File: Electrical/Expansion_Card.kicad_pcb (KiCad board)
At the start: 2 copper layers, 26 x 30 mm, 50 parts, among them J1 SJ-3501-SMT-TR, J2 SJ-3501-SMT-TR, P1 USB_C_Plug_USB2.0, U2 PCM2906, U3 TPA6132A2RTE, U4 LDLN050PUR, Y1 120-8-36B-CWY-TR

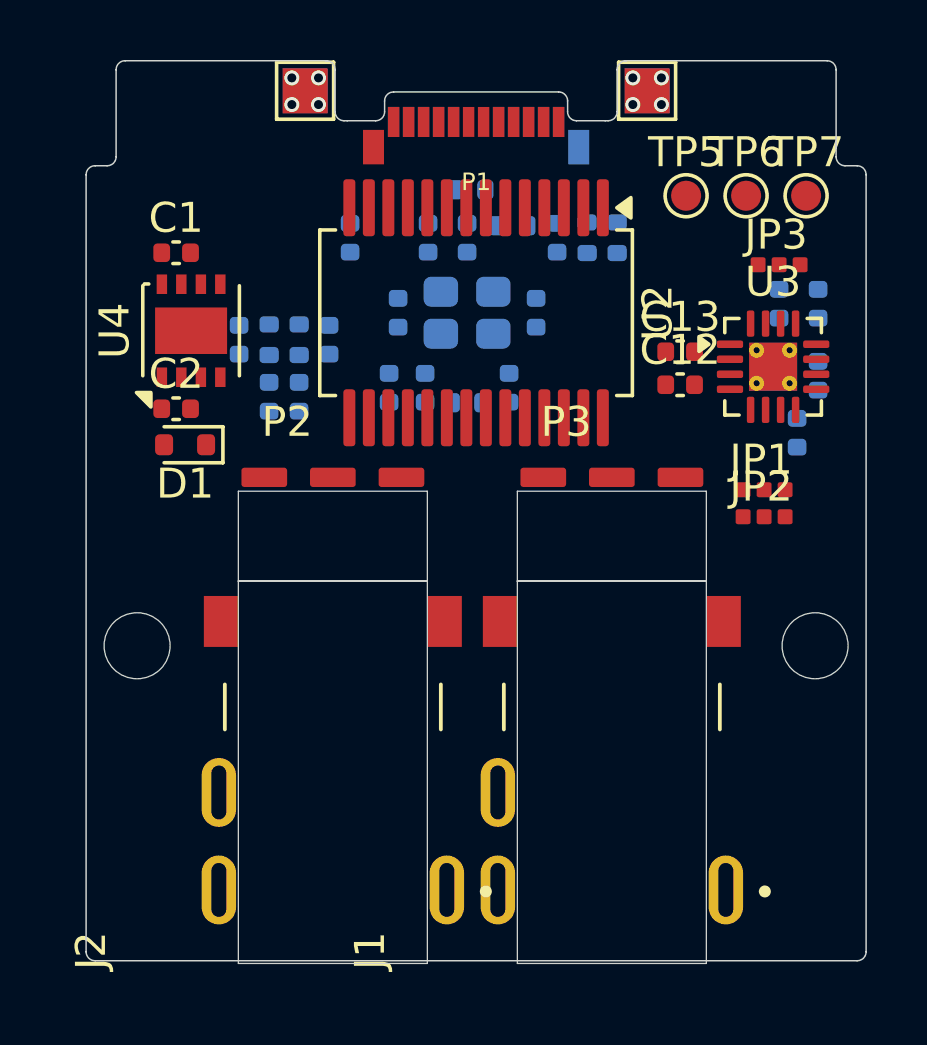
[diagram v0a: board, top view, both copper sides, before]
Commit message: Routing + output
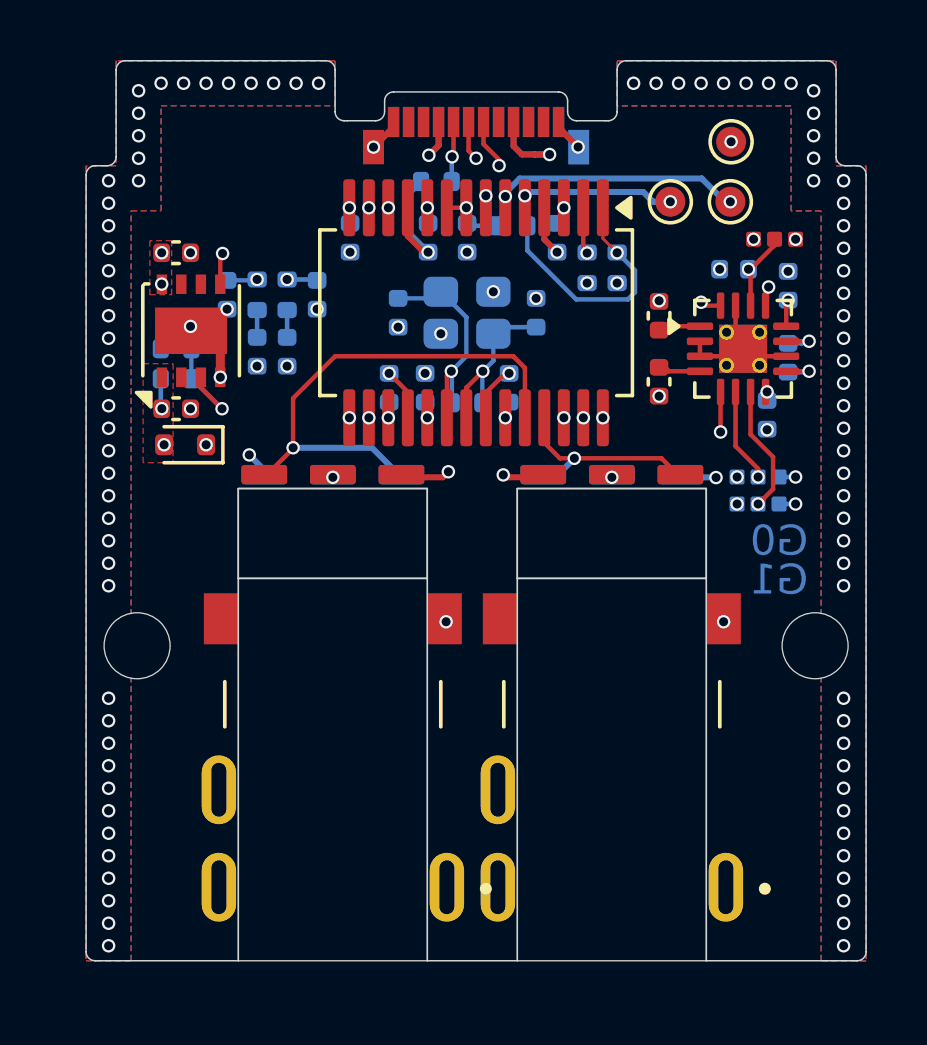
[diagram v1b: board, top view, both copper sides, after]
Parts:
- removed TP1, TP2, TP3, TP4: TestPoint, TestPoint:TestPoint_Pad_1.5x1.5mm
- added P4: ~, Expansion_Card:TX_RX_module, B.Cu at (144.5, 142.8)
- added P5: ~, Expansion_Card:TX_RX_module, B.Cu at (135.2, 142.8)
- added R6: 150k, Resistor_SMD:R_0402_1005Metric, B.Cu at (130.0, 136.6)
- added R9: 300k, Resistor_SMD:R_0402_1005Metric, B.Cu at (130.0, 137.6)
- JP1, JP2: moved to B.Cu
- moved TP7 3.08 mm to (148.5, 129.7)
- moved C17 1.89 mm to (148.6, 133.9), turned to 180 degrees
- moved C18 1.55 mm to (133.7, 136.7)
- moved C19 1.55 mm to (132.7, 136.7)
- moved C20 1.55 mm to (131.7, 134.8)
- moved C21 1.55 mm to (134.7, 134.8)
- moved R7 1.55 mm to (132.7, 134.8)
- moved R8 1.55 mm to (133.7, 134.8)
- moved C13 1.39 mm to (146.1, 135.5), turned to -90 degrees
- moved C14 1.17 mm to (149.7, 138.8)
- moved C15 1.17 mm to (150.4, 136.9)
- moved C16 1.17 mm to (150.4, 134.5)
- moved U3 1.17 mm to (148.9, 136.6)
- moved R1 1.16 mm to (138.7, 131.0), turned to 180 degrees
- moved R3 1.00 mm to (144.7, 133.9), turned to 90 degrees
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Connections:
- J1 pad 2: Net-(U3-OUTL) -> unconnected-(J1-Pad2)
- J2 pad 2: Net-(C18-Pad1) -> unconnected-(J2-Pad2)
- U4 pad 3: unconnected-(U4-FB-Pad3) -> Net-(U4-FB)
- Y1 pad 2: Net-(Y1-G-Pad2) -> GND
- Y1 pad 4: Net-(Y1-G-Pad2) -> GND
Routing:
- net /EN: track 0.00 -> 26.7 mm, vias 0 -> 3
- net GND: track 0.00 -> 26.1 mm, vias 8 -> 116
- net Net-(U3-OUTR): track 0.00 -> 19.4 mm, vias 0 -> 1
- net Net-(P2-OUT): track 0.00 -> 17.2 mm, vias 0 -> 1
- net VCCI: track 0.00 -> 15.6 mm, vias 0 -> 2
- net Net-(U2-VOUTL): track 0.00 -> 15.1 mm, vias 0 -> 2
- net Net-(C19-Pad1): track 0.00 -> 14.7 mm, vias 0 -> 1
- net Net-(U3-OUTL): track 0.00 -> 13.0 mm, vias 0 -> 2
- net Net-(U2-VOUTR): track 0.00 -> 12.5 mm, vias 0 -> 2
- net Net-(C18-Pad1): track 0.00 -> 12.2 mm, vias 0 -> 2
- net VDDI: track 0.00 -> 10.8 mm, vias 0 -> 2
- net Net-(U2-HID2): track 0.00 -> 9.45 mm, vias 0 -> 2
- net /USB_DP: track 0.00 -> 9.41 mm, vias 0 -> 2
- net Net-(U2-D+): track 0.00 -> 8.79 mm, vias 0 -> 1
- net Net-(U2-HID1): track 0.00 -> 8.14 mm, vias 0 -> 2
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- added copper zone on B.Cu, net GND
- added copper zone on F.Cu, net GND
- added copper zone on In1.Cu, net GND
- added copper zone on In3.Cu, net GND
- added copper zone on F.Cu, net VBUS
- added copper zone on In4.Cu, net VBUS
- added copper zone on F.Cu, net VCC
- added copper zone on In4.Cu, net VCC
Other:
- outline, holes or cut-outs redrawn
- copper layers 2 -> 6
- board text added: "G0"
- board text added: "G1"
- board text added: "RX"
- board text added: "TX"
